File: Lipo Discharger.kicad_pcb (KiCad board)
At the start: 2 copper layers, 160 x 110 mm, 122 parts, among them J2 USB_C_Receptacle_USB2.0_16P, J3 SWD, J4 XT60_P1, J5 XT60_P2, J6 XT60_P3, J7 XT60_P4, J8 XT60_P5, J9 FAN, Q1 IRLZ44N, Q2 IRLZ44N, Q3 IRLZ44N, Q4 IRLZ44N, Q5 IRLZ44N, Q6 2N2222, SW1 BOOT0_BTN, U1 MP2359DJ-LF-Z, U2 AMS1117-3.3, U3 STM32F103C8Tx, U4 PCA9685BS, Y1 8MHz

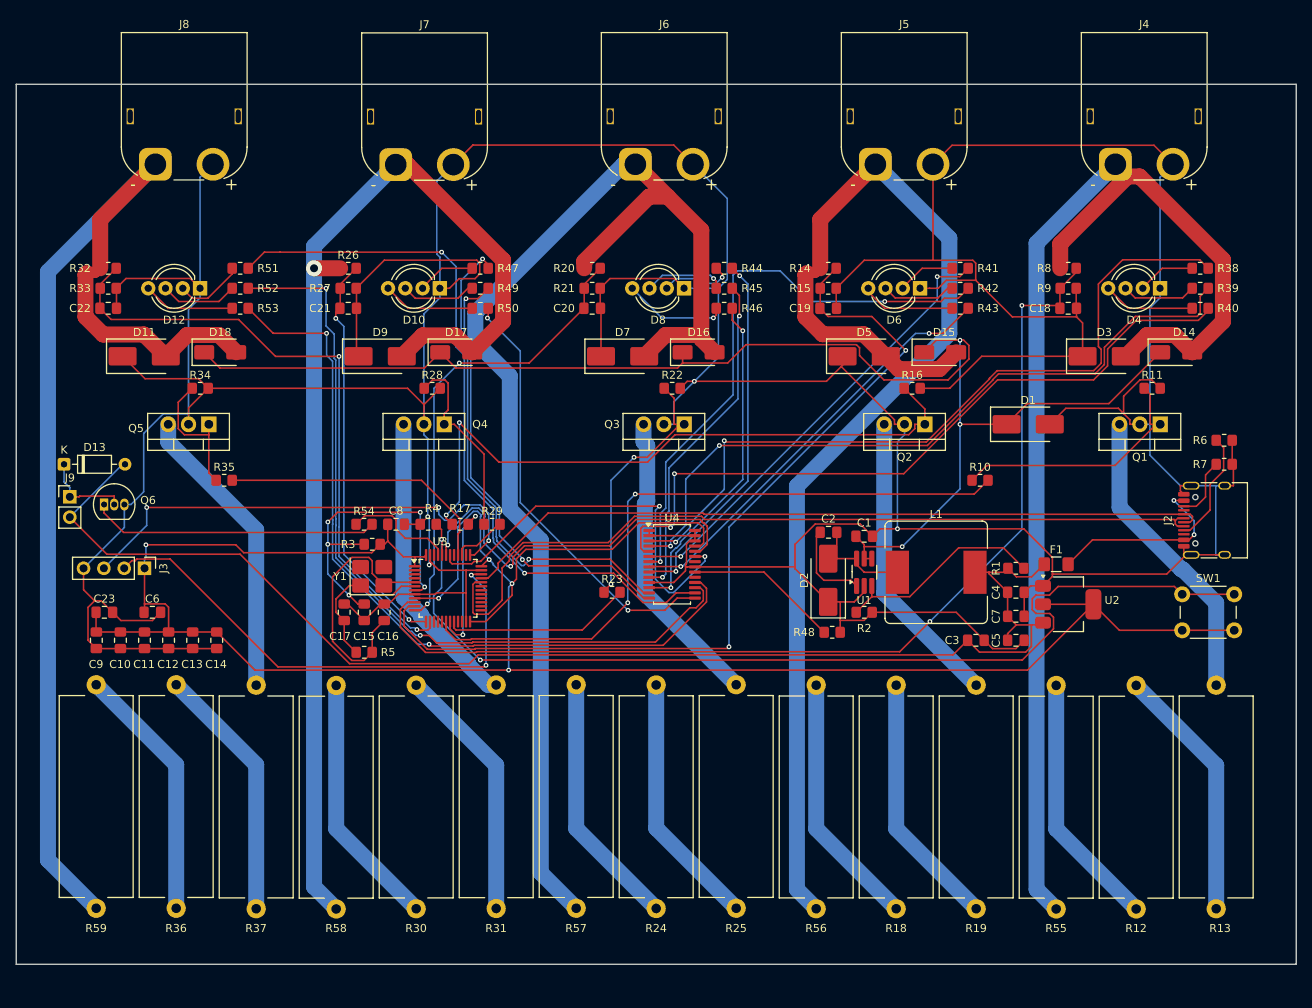
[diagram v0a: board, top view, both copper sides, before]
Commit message: Complete board redesign
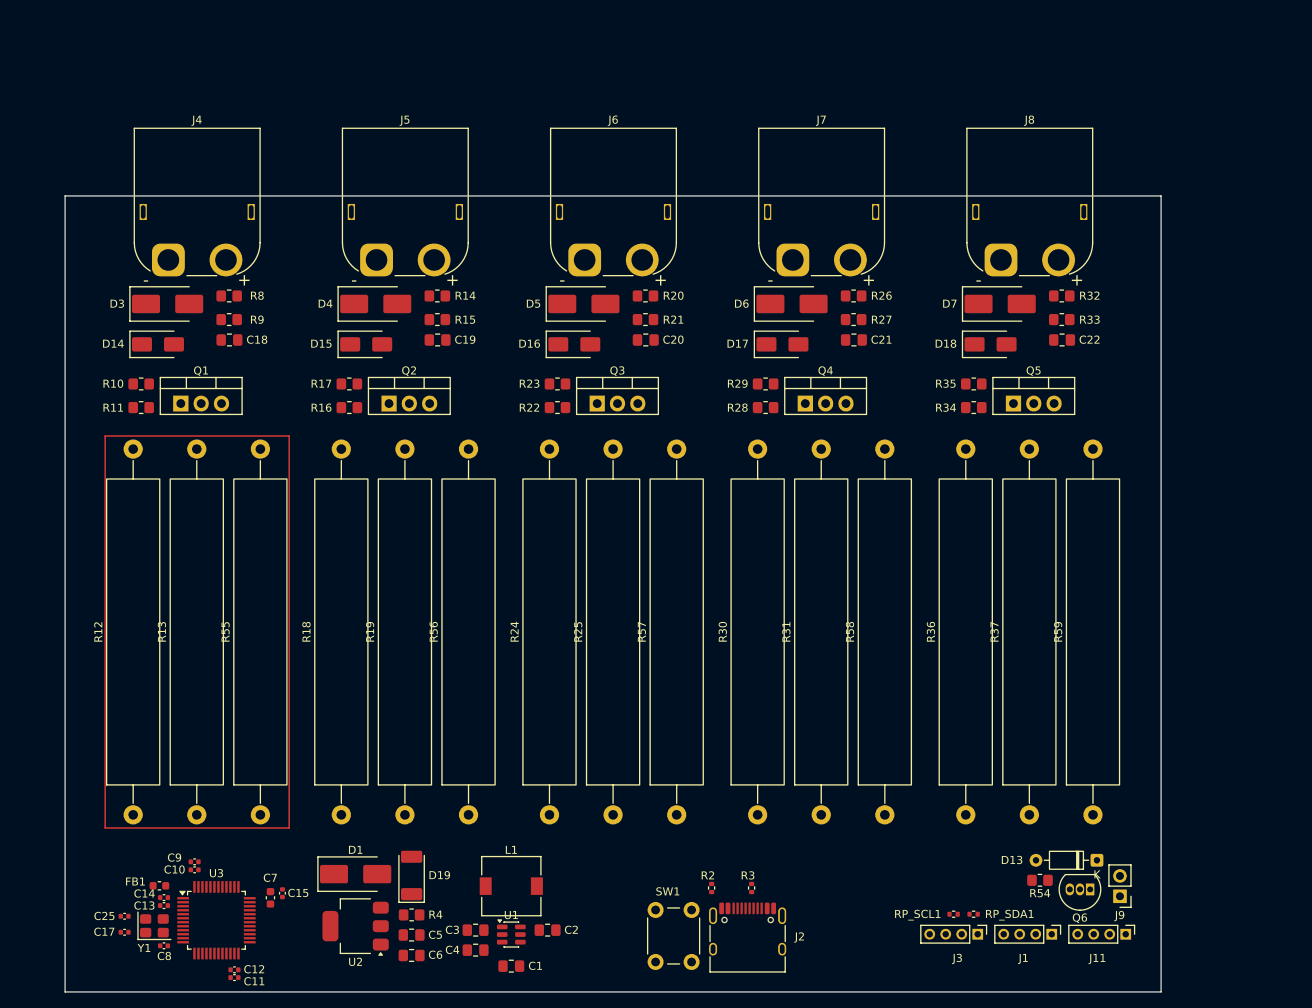
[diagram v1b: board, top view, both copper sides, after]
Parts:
- removed C16: 20pF, Capacitor_SMD:C_0805_2012Metric_Pad1.18x1.45mm_HandSolder
- removed C23: 100nF, Capacitor_SMD:C_0805_2012Metric_Pad1.18x1.45mm_HandSolder
- removed D10, D12, D8: LED_KRGB, LED_THT:LED_D5.0mm-4_RGB_Wide_Pins
- removed D11, D9: SMBJ26A, Diode_SMD:D_SMB_Handsoldering
- removed D2: SS34, Diode_SMD:D_SMB_Handsoldering
- removed F1: Polyfuse, Fuse:Fuse_1206_3216Metric_Pad1.42x1.75mm_HandSolder
- removed R1: 100k, Resistor_SMD:R_0805_2012Metric_Pad1.20x1.40mm_HandSolder
- removed R38, R41, R44, R47, R51: 68, Resistor_SMD:R_0805_2012Metric_Pad1.20x1.40mm_HandSolder
- removed R39, R40, R42, R43, R45, R46, R49, R50, R52, R53: 22, Resistor_SMD:R_0805_2012Metric_Pad1.20x1.40mm_HandSolder
- removed R48: 10k, Resistor_SMD:R_0805_2012Metric_Pad1.20x1.40mm_HandSolder
- removed R5: 1M, Resistor_SMD:R_0805_2012Metric_Pad1.20x1.40mm_HandSolder
- removed R6, R7: 5.1k, Resistor_SMD:R_0805_2012Metric_Pad1.20x1.40mm_HandSolder
- removed U4: PCA9685BS, Package_SO:TSSOP-28_4.4x9.7mm_P0.65mm
- added C25: 10p, Capacitor_SMD:C_0402_1005Metric, F.Cu at (25.6, 116.0)
- added D19: LED, LED_SMD:LED_2010_5025Metric_Pad1.52x2.65mm_HandSolder, F.Cu at (61.4, 110.9)
- added FB1: 120R, Inductor_SMD:L_0603_1608Metric, F.Cu at (29.9, 112.2)
- added J1: Conn_01x04_Male, Connector_PinHeader_2.00mm:PinHeader_1x04_P2.00mm_Vertical, F.Cu at (141.5, 118.2)
- added J11: Conn_01x04_Male, Connector_PinHeader_2.00mm:PinHeader_1x04_P2.00mm_Vertical, F.Cu at (150.7, 118.2)
- added RP_SCL1: 2k2, Resistor_SMD:R_0402_1005Metric, F.Cu at (129.2, 115.7)
- added RP_SDA1: 2k2, Resistor_SMD:R_0402_1005Metric, F.Cu at (131.7, 115.7)
- C10, C11, C12, C8, C9: value 100nF -> 100n; footprint Capacitor_SMD:C_0805_2012Metric_Pad1.18x1.45mm_HandSolder -> Capacitor_SMD:C_0402_1005Metric
- C13: value 1uF -> 10n; footprint Capacitor_SMD:C_0805_2012Metric_Pad1.18x1.45mm_HandSolder -> Capacitor_SMD:C_0402_1005Metric
- C14: value 10nF -> 1u; footprint Capacitor_SMD:C_0805_2012Metric_Pad1.18x1.45mm_HandSolder -> Capacitor_SMD:C_0402_1005Metric
- C15: value 100nF -> 1u; footprint Capacitor_SMD:C_0805_2012Metric_Pad1.18x1.45mm_HandSolder -> Capacitor_SMD:C_0402_1005Metric
- C17: value 20pF -> 10p; footprint Capacitor_SMD:C_0805_2012Metric_Pad1.18x1.45mm_HandSolder -> Capacitor_SMD:C_0402_1005Metric
- C3, C4: value 22uF 10V -> 22µF
- C5: value 10uF -> 10µF
- C6: value 10uF -> 22µF
- C7: value 100nF -> 10u; footprint Capacitor_SMD:C_0805_2012Metric_Pad1.18x1.45mm_HandSolder -> Capacitor_SMD:C_0603_1608Metric
- D1: value D_TVS -> SS34
- D4, D6: value LED_KRGB -> SMBJ26A; footprint LED_THT:LED_D5.0mm-4_RGB_Wide_Pins -> Diode_SMD:D_SMB_Handsoldering
- J3: value SWD -> Conn_01x04_Male; footprint Connector_PinHeader_2.54mm:PinHeader_1x04_P2.54mm_Vertical -> Connector_PinHeader_2.00mm:PinHeader_1x04_P2.00mm_Vertical
- J5: value XT60_P2 -> XT60_P1
- J6: value XT60_P3 -> XT60_P1
- J7: value XT60_P4 -> XT60_P1
- J8: value XT60_P5 -> XT60_P1
- L1: value 22uH -> 4.7µH; footprint Inductor_SMD:L_Bourns_SRR1260 -> Inductor_SMD:L_7.3x7.3_H4.5
- R12, R13, R18, R19, R24, R25, R30, R31, R36, R37, R55, R56, R57, R58, R59: footprint Resistor_THT:R_Axial_Power_L25.0mm_W9.0mm_P27.94mm -> Resistor_THT:R_Axial_Power_L38.0mm_W6.4mm_P45.72mm
- R15, R21, R27, R33, R9: value 150k -> 120k
- R2: value 20k -> 10k; footprint Resistor_SMD:R_0805_2012Metric_Pad1.20x1.40mm_HandSolder -> Resistor_SMD:R_0402_1005Metric
- R3: value 10k -> 1k5; footprint Resistor_SMD:R_0805_2012Metric_Pad1.20x1.40mm_HandSolder -> Resistor_SMD:R_0402_1005Metric
- R4: value 10k -> 1K
- SW1: value BOOT0_BTN -> SW_Push
- U1: value MP2359DJ-LF-Z -> AP63205WU-7; footprint Package_TO_SOT_SMD:TSOT-23-6_HandSoldering -> Package_TO_SOT_SMD:TSOT-23-6
- U3: value STM32F103C8Tx -> STM32F103C8T6
- Y1: value 8MHz -> 16MHz; footprint Crystal:Crystal_SMD_3225-4Pin_3.2x2.5mm_HandSoldering -> Crystal:Crystal_SMD_3225-4Pin_3.2x2.5mm
- moved J9 140.4 mm to (150.0, 113.5), turned to 180 degrees
- moved D13 138.3 mm to (147.1, 109.0), turned to 180 degrees
- moved Q6 132.3 mm to (146.3, 112.6), turned to 180 degrees
- moved R13 128.0 mm to (34.6, 103.3)
- moved D14 127.3 mm to (29.7, 44.5)
- moved R11 126.4 mm to (27.6, 52.4)
- moved R12 125.9 mm to (26.6, 103.3)
- moved R59 125.1 mm to (146.6, 103.3)
- moved Q1 122.4 mm to (32.6, 51.9), turned to 0 degrees
- moved C22 119.3 mm to (142.8, 44.0)
- moved R33 119.3 mm to (142.7, 41.4)
- moved R32 119.2 mm to (142.7, 38.5)
- moved J4 119.0 mm to (31.0, 34.0)
- moved D3 117.3 mm to (30.9, 39.5)
- moved J3 113.8 mm to (132.2, 118.2)
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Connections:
- net USB_DM renamed /STM32/USB_D-
- C1 pad 2: -BATT -> GND
- C10 pad 1: -BATT -> +3.3V
- C10 pad 2: +3.3V -> GND
- C11 pad 1: -BATT -> +3.3V
- C11 pad 2: +3.3V -> GND
- C12 pad 1: -BATT -> +3.3V
- C12 pad 2: +3.3V -> GND
- C13 pad 1: -BATT -> Net-(U3-VDDA)
- C13 pad 2: +3.3V -> GND
- C14 pad 1: -BATT -> Net-(U3-VDDA)
- C14 pad 2: +3.3V -> GND
- C15 pad 1: -BATT -> +3.3V
- C15 pad 2: Net-(U3-NRST) -> GND
- C17 pad 1: Net-(U3-PD1) -> /STM32/HSE_IN
- C17 pad 2: -BATT -> GND
- C18 pad 2: -BATT -> GND
- C19 pad 2: -BATT -> GND
- C2 pad 1: Net-(U1-BST) (its old number) -> Net-(U1-SW)
- C20 pad 2: -BATT -> GND
- C21 pad 2: -BATT -> GND
- C22 pad 2: -BATT -> GND
- C3 pad 2: -BATT -> GND
- C4 pad 2: -BATT -> GND
- C5 pad 2: -BATT -> GND
- C6 pad 2: -BATT -> GND
- C7 pad 1: +5V -> +3.3V
- C7 pad 2: -BATT -> GND
- C8 pad 1: +3.3V -> /STM32/NRST
- C8 pad 2: -BATT -> GND
- C9 pad 1: -BATT -> +3.3V
- C9 pad 2: +3.3V -> GND
- D1 pad 1: +BATT -> +5V
- D1 pad 2: -BATT -> +3.3V
- D14 pad 2: VBAT_P1 -> Net-(D14-A)
- D15 pad 2: VBAT_P2 -> Net-(D15-A)
- D16 pad 2: VBAT_P3 -> Net-(D16-A)
- D17 pad 2: VBAT_P4 -> Net-(D17-A)
- D18 pad 2: VBAT_P5 -> Net-(D18-A)
- D3 pad 1: -BATT -> GND
- D3 pad 2: VBAT_P1 -> Net-(D14-A)
- D4 pad 1: -BATT -> GND
- D4 pad 2: Net-(D4-RA) -> Net-(D15-A)
- D5 pad 1: -BATT -> GND
- D5 pad 2: VBAT_P2 -> Net-(D16-A)
- D6 pad 1: -BATT -> GND
- D6 pad 2: Net-(D6-RA) -> Net-(D17-A)
- D7 pad 1: -BATT -> GND
- D7 pad 2: VBAT_P3 -> Net-(D18-A)
- J2 pad A1: -BATT -> GND
- J2 pad A12: -BATT -> GND
- J2 pad A4: Net-(F1-Pad2) -> +5V
- J2 pad A5: Net-(J2-CC1) -> unconnected-(J2-CC1-PadA5)
- J2 pad A6: USB_DP -> /STM32/USB_D+
- J2 pad A9: Net-(F1-Pad2) -> +5V
- J2 pad B1: -BATT -> GND
- J2 pad B12: -BATT -> GND
- J2 pad B4: Net-(F1-Pad2) -> +5V
- J2 pad B5: Net-(J2-CC2) -> unconnected-(J2-CC2-PadB5)
- J2 pad B6: USB_DP -> /STM32/USB_D+
- J2 pad B9: Net-(F1-Pad2) -> +5V
- J2 pad SH: -BATT -> unconnected-(J2-SHIELD-PadSH)_1
- J3 pad 2: Net-(J3-Pin_2) -> /STM32/I2C2_SCL
- J3 pad 3: Net-(J3-Pin_3) -> /STM32/I2C2_SDA
- J3 pad 4: -BATT -> GND
- J4 pad 1: VBAT_P1 -> GND
- J4 pad 2: -BATT -> Net-(D14-A)
- J5 pad 1: VBAT_P2 -> GND
- J5 pad 2: -BATT -> Net-(D15-A)
- J6 pad 1: VBAT_P3 -> GND
- J6 pad 2: -BATT -> Net-(D16-A)
- J7 pad 1: VBAT_P4 -> GND
- J7 pad 2: -BATT -> Net-(D17-A)
- J8 pad 1: VBAT_P5 -> GND
- J8 pad 2: -BATT -> Net-(D18-A)
- Q1 pad 2: -BATT -> GND
- Q2 pad 2: -BATT -> GND
- Q3 pad 2: -BATT -> GND
- Q4 pad 2: -BATT -> GND
- Q5 pad 2: -BATT -> GND
- Q6 pad 3: -BATT -> GND
- R11 pad 2: -BATT -> GND
- R14 pad 1: VBAT_P2 -> Net-(D15-A)
- R15 pad 2: -BATT -> GND
- R16 pad 2: -BATT -> GND
- R2 pad 1: Net-(U1-FB) -> GND
- R2 pad 2: -BATT -> Net-(U3-BOOT0)
- R20 pad 1: VBAT_P3 -> Net-(D16-A)
- R21 pad 2: -BATT -> GND
- R22 pad 2: -BATT -> GND
- R26 pad 1: VBAT_P4 -> Net-(D17-A)
- R27 pad 2: -BATT -> GND
- R28 pad 2: -BATT -> GND
- R3 pad 2: Net-(U3-NRST) -> /STM32/USB_D+
- R32 pad 1: VBAT_P5 -> Net-(D18-A)
- R33 pad 2: -BATT -> GND
- R34 pad 2: -BATT -> GND
- R4 pad 1: Net-(U3-BOOT0) -> Net-(D19-K)
- R4 pad 2: -BATT -> GND
- R55 pad 1: VBAT_P1 -> Net-(R12-Pad1)
- R55 pad 2: Net-(R12-Pad1) -> Net-(D14-A)
- R56 pad 1: VBAT_P2 -> Net-(R18-Pad1)
- R56 pad 2: Net-(R18-Pad1) -> Net-(D15-A)
- R57 pad 1: VBAT_P3 -> Net-(R24-Pad1)
- R57 pad 2: Net-(R24-Pad1) -> Net-(D16-A)
- R58 pad 1: VBAT_P4 -> Net-(R30-Pad1)
- R58 pad 2: Net-(R30-Pad1) -> Net-(D17-A)
- R59 pad 1: VBAT_P5 -> Net-(R36-Pad1)
- R59 pad 2: Net-(R36-Pad1) -> Net-(D18-A)
- R8 pad 1: VBAT_P1 -> Net-(D14-A)
- R9 pad 2: -BATT -> GND
- SW1 pad 1: Net-(U3-BOOT0) -> +3.3V
- SW1 pad 2: +3.3V -> Net-(U3-BOOT0)
- U1 pad 1: Net-(U1-BST) (its old number) -> +5V
- U1 pad 2: -BATT -> +BATT
- U1 pad 3: Net-(U1-FB) -> +BATT
- U1 pad 4: +BATT -> GND
- U1 pad 5: +BATT -> Net-(U1-SW)
- U2 pad 1: -BATT -> GND
- U3 pad 15: unconnected-(U3-PA5-Pad15) -> GATE_P1
- U3 pad 16: unconnected-(U3-PA6-Pad16) -> GATE_P2
- U3 pad 17: unconnected-(U3-PA7-Pad17) -> GATE_P3
- U3 pad 18: GATE_P1 -> unconnected-(U3-PB0-Pad18)
- U3 pad 19: GATE_P2 -> unconnected-(U3-PB1-Pad19)
- U3 pad 20: GATE_P3 -> unconnected-(U3-PB2-Pad20)
- U3 pad 21: unconnected-(U3-PB10-Pad21) -> /STM32/I2C2_SCL
- U3 pad 22: unconnected-(U3-PB11-Pad22) -> /STM32/I2C2_SDA
- U3 pad 23: -BATT -> GND
- U3 pad 29: unconnected-(U3-PA8-Pad29) -> GATE_P4
- U3 pad 30: unconnected-(U3-PA9-Pad30) -> GATE_P5
- U3 pad 31: unconnected-(U3-PA10-Pad31) -> FAN_CTRL
- U3 pad 33: USB_DP -> /STM32/USB_D+
- U3 pad 34: Net-(J3-Pin_2) -> /STM32/SWDIO
- U3 pad 35: -BATT -> GND
- U3 pad 37: Net-(J3-Pin_3) -> /STM32/SWCLK
- U3 pad 39: GATE_P4 -> unconnected-(U3-PB3-Pad39)
- U3 pad 40: GATE_P5 -> unconnected-(U3-PB4-Pad40)
- U3 pad 42: I2C_SCL -> /STM32/USART1_TX
- U3 pad 43: I2C_SDA -> /STM32/USART1_RX
- U3 pad 45: FAN_CTRL -> unconnected-(U3-PB8-Pad45)
- U3 pad 47: -BATT -> GND
- U3 pad 5: Net-(U3-PD0) -> /STM32/HSE_IN
- U3 pad 6: Net-(U3-PD1) -> /STM32/HSE_OUT
- U3 pad 7: Net-(U3-NRST) -> /STM32/NRST
- U3 pad 8: -BATT -> GND
- U3 pad 9: +3.3V -> Net-(U3-VDDA)
- Y1 pad 1: Net-(U3-PD1) -> /STM32/HSE_IN
- Y1 pad 2: Net-(U3-PD0) -> GND
- Y1 pad 3: (no net) -> /STM32/HSE_OUT
- Y1 pad 4: (no net) -> GND
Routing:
- net -BATT: track 779.2 -> 0.00 mm, vias 4 -> 0
- net +3.3V: track 292.2 -> 0.00 mm, vias 5 -> 0
- net +BATT: track 178.7 -> 0.00 mm, vias 3 -> 0
- net +5V: track 166.0 -> 0.00 mm
- net VBAT_P3: track 157.9 -> 0.00 mm
- net VBAT_P1: track 155.0 -> 0.00 mm
- net VBAT_P2: track 151.5 -> 0.00 mm
- net VBAT_P5: track 147.3 -> 0.00 mm
- net VBAT_P4: track 143.9 -> 0.00 mm, vias 1 -> 0
- net ADC_P1: track 128.5 -> 0.00 mm, vias 2 -> 0
- net Net-(U3-BOOT0): track 127.5 -> 0.00 mm, vias 2 -> 0
- net ADC_P2: track 110.4 -> 0.00 mm, vias 2 -> 0
- net /STM32/USB_D-: track 103.3 -> 0.00 mm
- net LED_P5_G: track 98.9 -> 0.00 mm, vias 2 -> 0
- net LED_P5_B: track 96.6 -> 0.00 mm, vias 2 -> 0
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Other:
- board size 160 x 110 mm -> 137 x 99.5 mm
